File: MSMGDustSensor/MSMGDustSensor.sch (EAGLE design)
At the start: 55 parts, among them J2 POWER_JACK, Q1 BC817-16LT1SMD, U1 MCP6002-SO8, U2 TSL2591, U3 BME280BOARD, U4 BME280, U6 BUZZER, X1 53261-0871, X2 5268-02

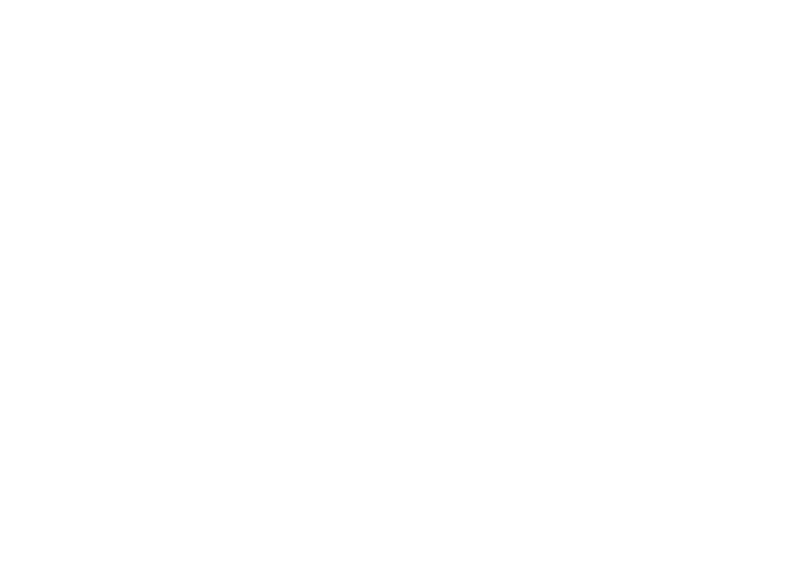
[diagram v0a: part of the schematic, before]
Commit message: almost done
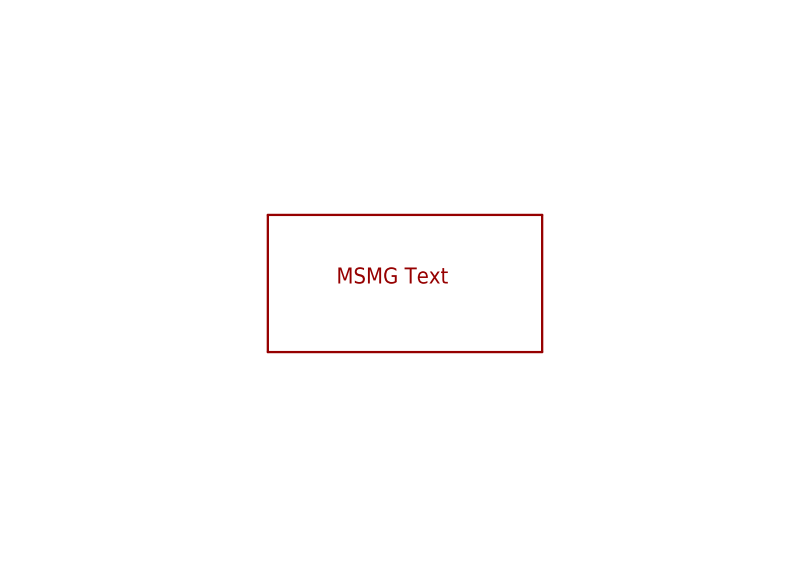
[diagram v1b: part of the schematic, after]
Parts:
- added U$1: MSMG_TEXT, MSMG:MSMG_TEXT
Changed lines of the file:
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@@
 <part name="X2" library="OSSI" deviceset="5268-02" device=""/>
 <part name="GND28" library="MSMG" deviceset="GND" device=""/>
+<part name="U$1" library="MSMG" deviceset="MSMG_TEXT" device=""/>
 </parts>
 <sheets>
@@
 <instance part="X2" gate="G$1" x="27.94" y="246.38" rot="R180"/>
 <instance part="GND28" gate="1" x="35.56" y="238.76"/>
+<instance part="U$1" gate="G$1" x="233.68" y="58.42"/>
 </instances>
 <busses>
